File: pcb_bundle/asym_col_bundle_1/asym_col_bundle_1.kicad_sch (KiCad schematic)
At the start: 43 parts

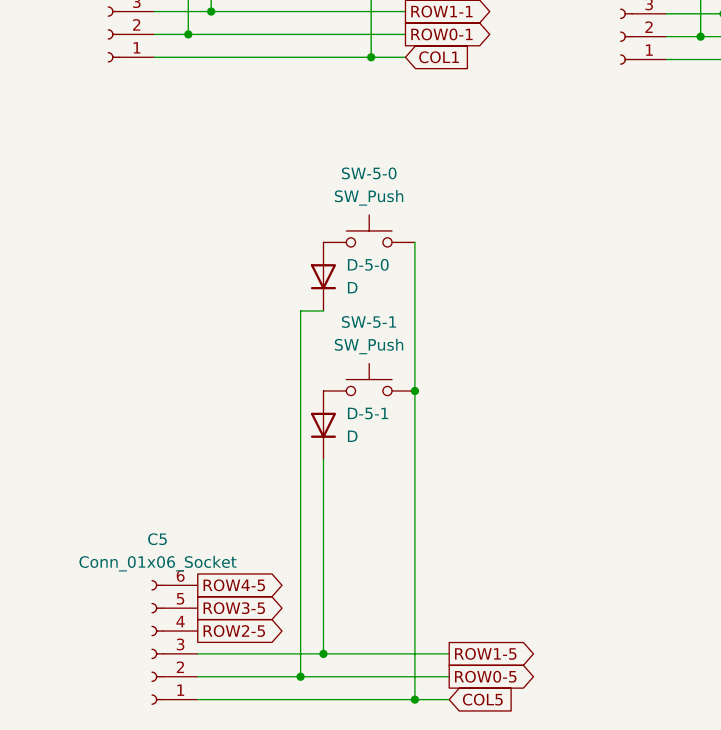
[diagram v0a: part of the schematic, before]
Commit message: [unstable] interim state
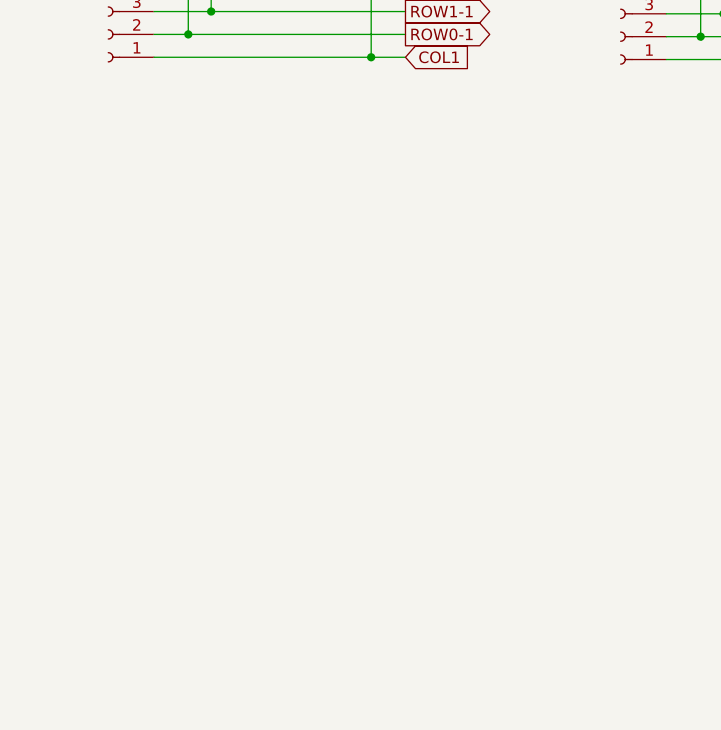
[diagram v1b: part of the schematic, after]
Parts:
- removed C5: Conn_01x06_Socket, Connector_JST:JST_PH_S6B-PH-K_1x06_P2.00mm_Horizontal, symbol Connector:Conn_01x06_Socket
- removed D-5-0, D-5-1: D, crustrusk:Diode_TH_SMD_REVERSIBLE, symbol Device:D
- removed SW-5-0, SW-5-1: SW_Push, crustrusk:Kailh_socket_MX, symbol Switch:SW_Push
